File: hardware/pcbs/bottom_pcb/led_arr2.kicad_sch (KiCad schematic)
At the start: 107 parts, among them U10 TPIC6C595, U3 TPIC6C595, U4 TPIC6C595, U5 TPIC6C595, U6 TPIC6C595, U7 TPIC6C595, U8 TPIC6C595, U9 TPIC6C595

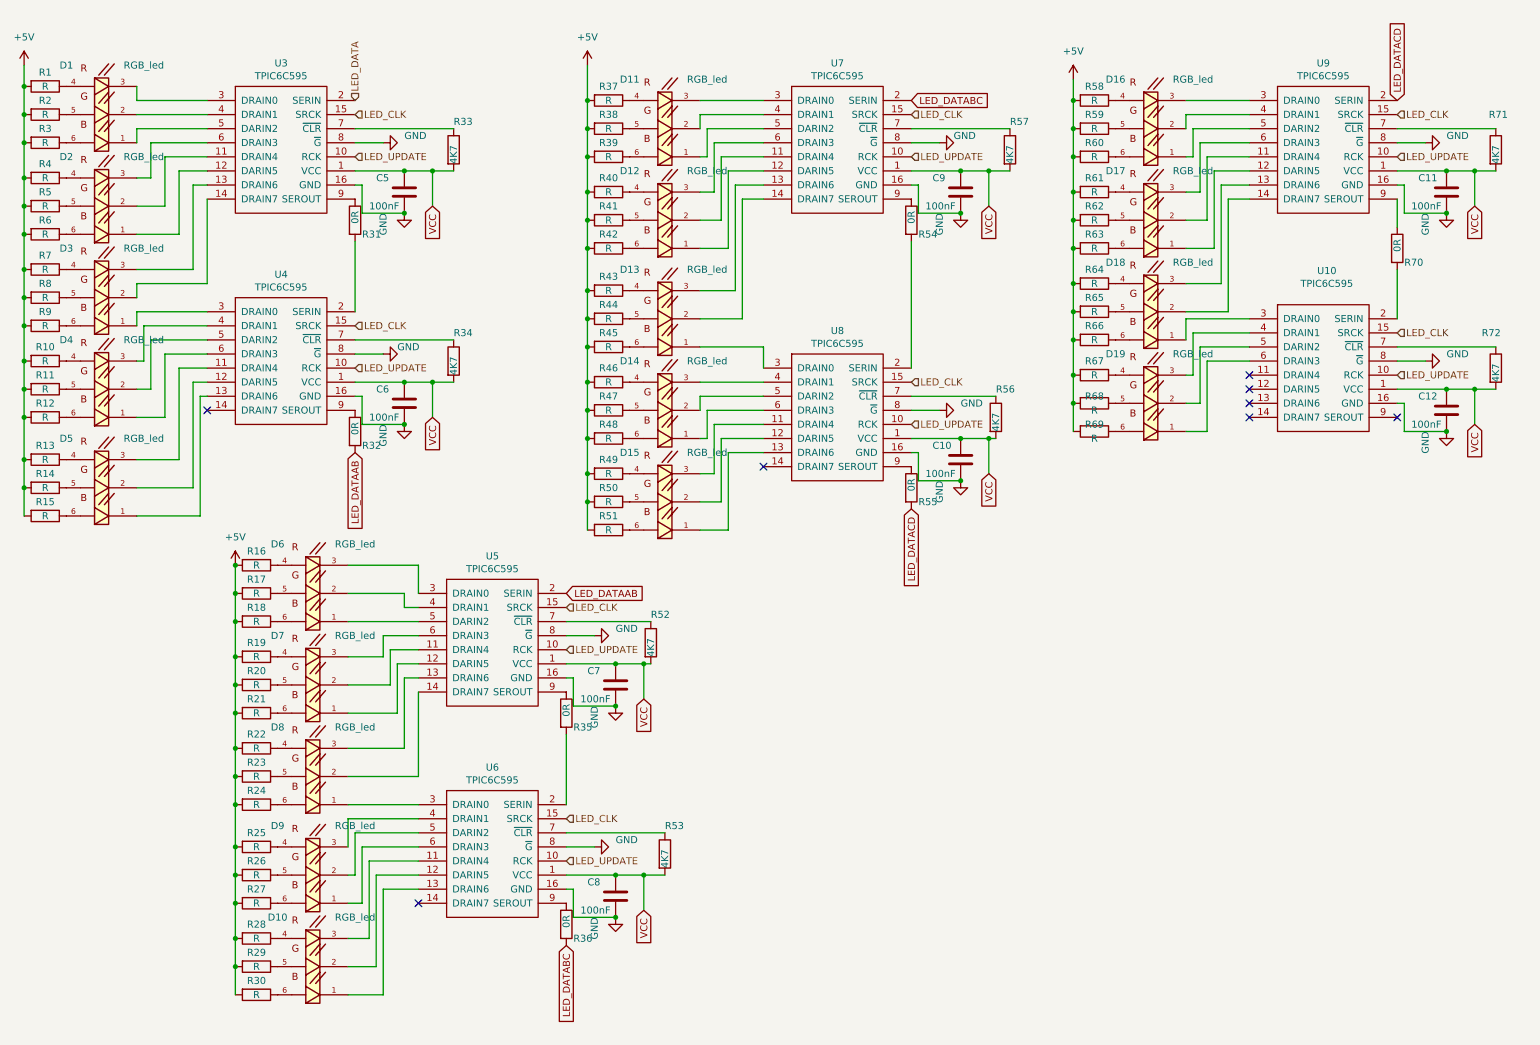
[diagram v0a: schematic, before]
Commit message: pcb main fertig
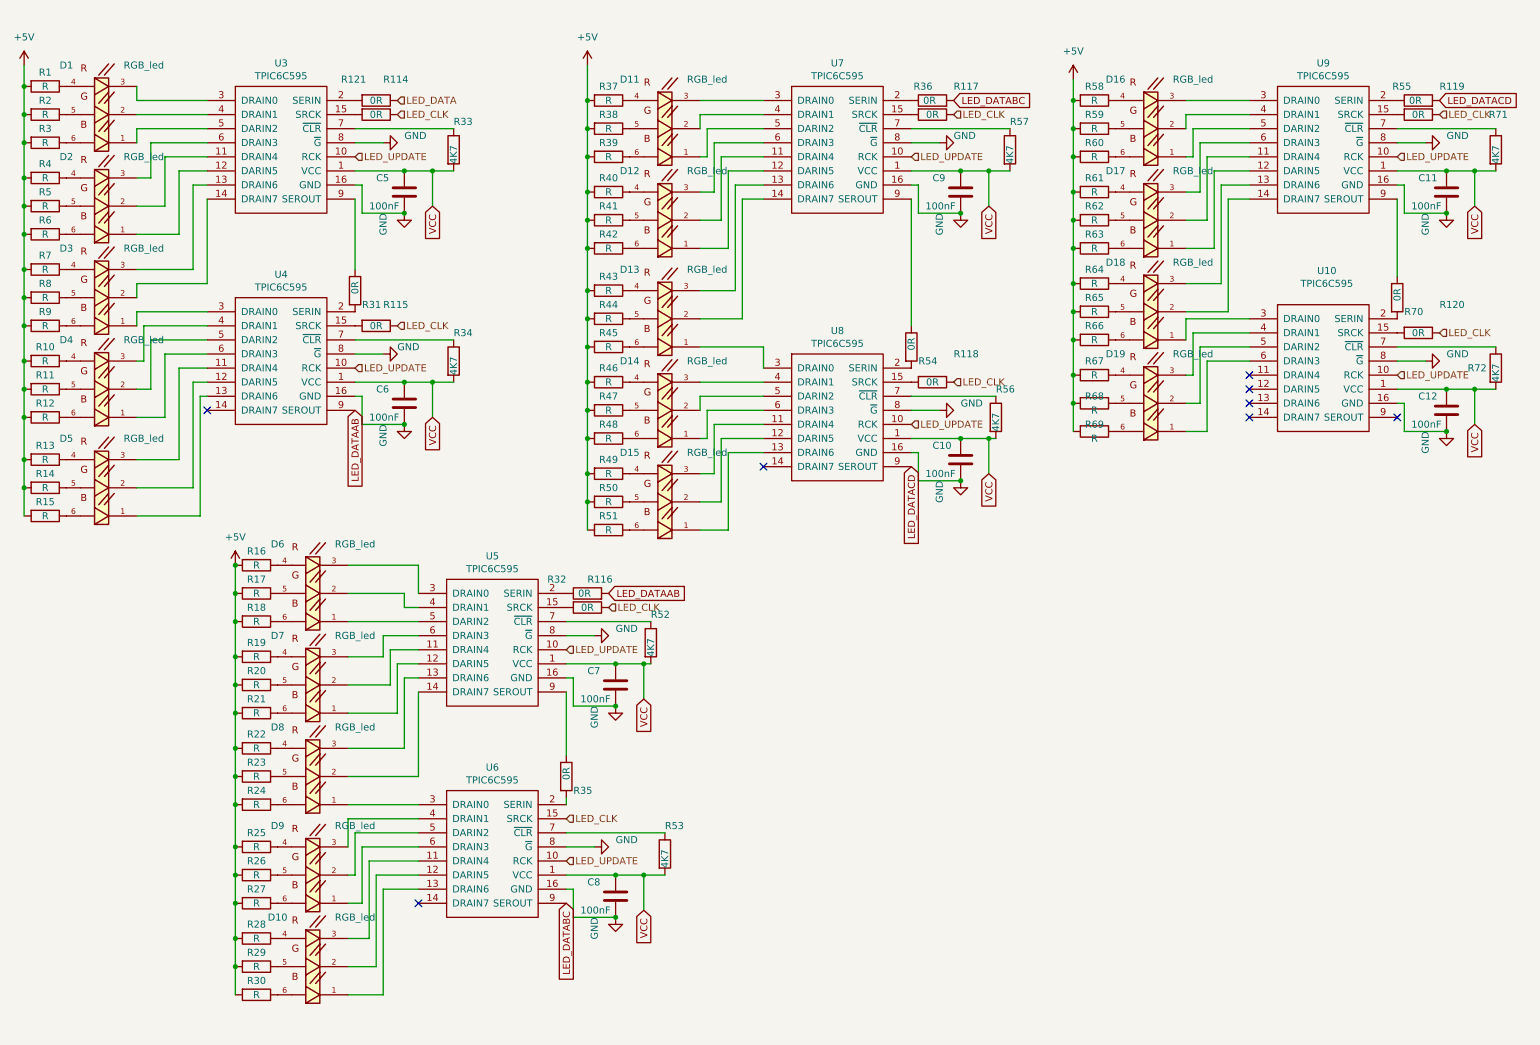
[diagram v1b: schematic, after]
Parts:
- added R114, R115, R116, R117, R118, R119, R120, R121: 0R, Resistor_SMD:R_1206_3216Metric_Pad1.30x1.75mm_HandSolder, symbol Device:R
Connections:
- net LED_CLK: now also R114.1, R115.1, R116.1, R117.1, R118.1, R119.1, R120.1; no longer U10.15 (SRCK), U3.15 (SRCK), U4.15 (SRCK), U5.15 (SRCK), U7.15 (SRCK), U8.15 (SRCK), U9.15 (SRCK)
- net LED_DATA: now also R121.1; no longer U3.2 (SERIN)
- net LED_DATAAB: now also U4.9 (SEROUT); no longer U5.2 (SERIN)
- net LED_DATABC: now also U6.9 (SEROUT); no longer U7.2 (SERIN)
- net LED_DATACD: now also U8.9 (SEROUT); no longer U9.2 (SERIN)
- net at R36.1: now also U7.2 (SERIN); no longer U6.9 (SEROUT)
- net at R55.1: now also U9.2 (SERIN); no longer U8.9 (SEROUT)
- net at R32.1: now also U5.2 (SERIN); no longer U4.9 (SEROUT)
- new net: R116.2, U5.15 (SRCK)
- new net: R119.2, U9.15 (SRCK)
- new net: R118.2, U8.15 (SRCK)
- new net: R121.2, U3.2 (SERIN)
- new net: R114.2, U3.15 (SRCK)
- new net: R120.2, U10.15 (SRCK)
- new net: R117.2, U7.15 (SRCK)
- new net: R115.2, U4.15 (SRCK)
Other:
- moved on the sheet: R31, R32, R35, R36, R54, R55, R70
